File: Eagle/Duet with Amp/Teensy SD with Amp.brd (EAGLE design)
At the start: 34.3 x 63.2 mm, 20 parts, among them IC1 LM386N-4

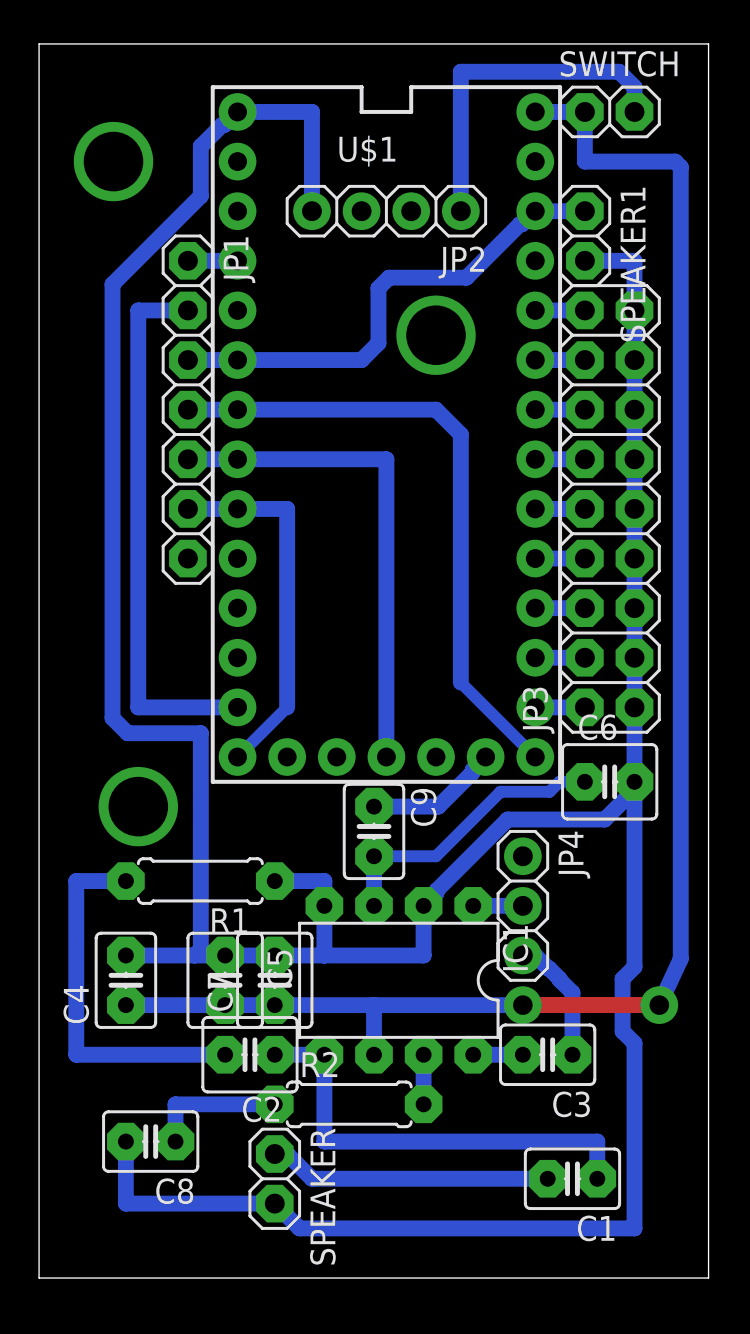
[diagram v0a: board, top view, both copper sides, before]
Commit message: Traced to 32mils
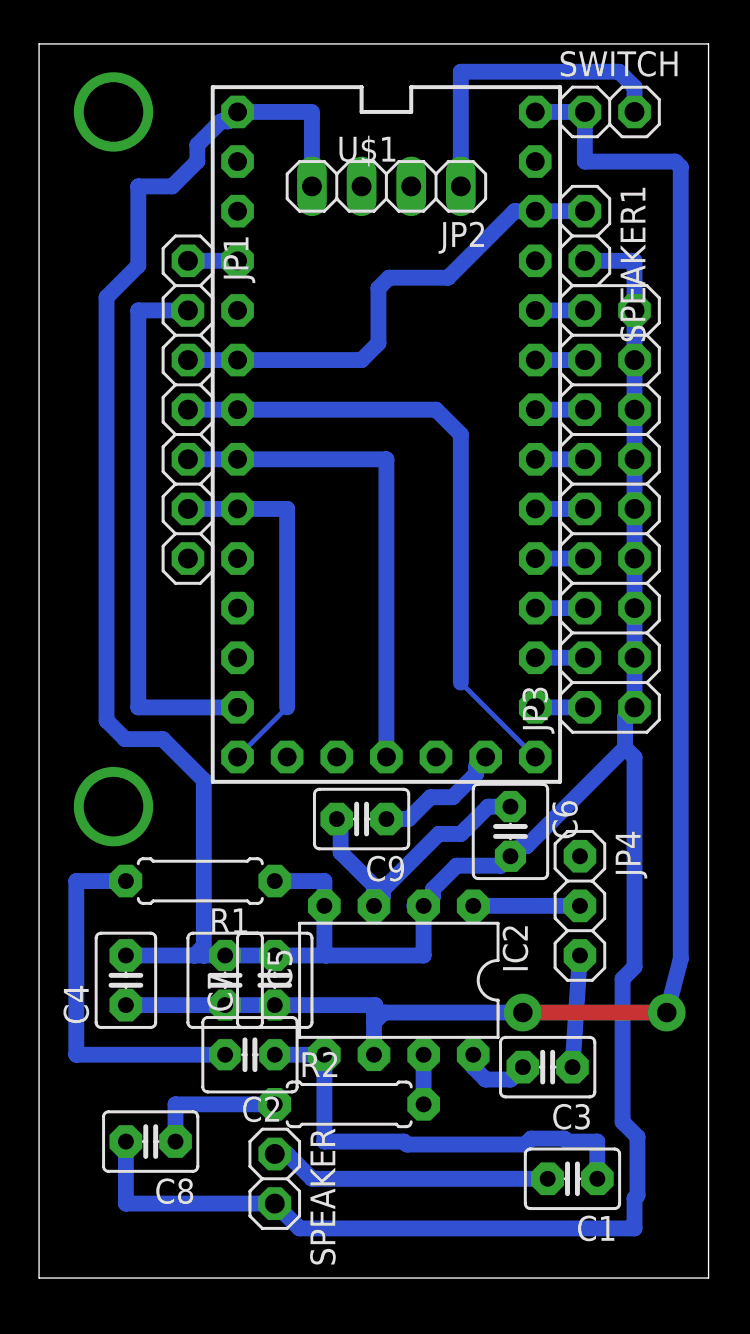
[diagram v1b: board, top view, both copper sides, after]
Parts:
- IC2: value LM386N-4 -> LM386N-1
- moved C6 5.68 mm to (24.1, 22.9), turned to 270 degrees
- moved JP4 2.92 mm to (27.7, 19.1)
- moved JP2 1.27 mm to (17.8, 55.9)
- moved C9 0.90 mm to (16.5, 23.5), turned to 180 degrees
- moved C3 0.63 mm to (26.0, 10.8)
- renumbered IC1 to IC2
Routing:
- net N$26: track 2.54 -> 5.46 mm
- net GND: track 204.2 -> 205.7 mm
- net N$2: track 2.54 -> 3.70 mm
- net N$1: track 6.53 -> 5.73 mm
- net N$6: track 14.9 -> 15.5 mm

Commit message: Revert "Traced to 32mils"
This reverts commit ffbe95997752b5ed6823b856a1fed8613c21e4f0.
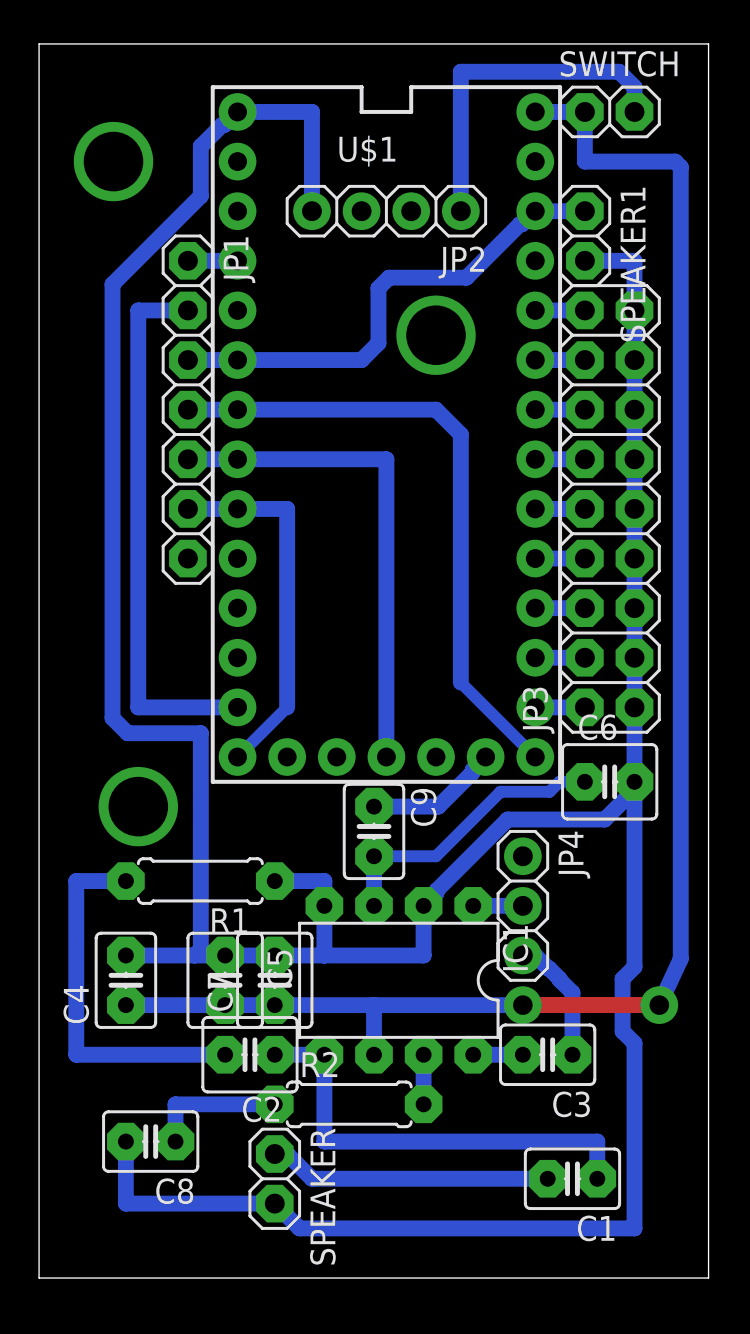
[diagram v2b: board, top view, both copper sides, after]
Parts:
- IC1: value LM386N-1 -> LM386N-4
- moved C6 5.68 mm to (29.2, 25.4), turned to 0 degrees
- moved JP4 2.92 mm to (24.8, 19.1)
- moved JP2 1.27 mm to (17.8, 54.6)
- moved C9 0.90 mm to (17.1, 22.9), turned to 270 degrees
- moved C3 0.63 mm to (26.0, 11.4)
- renumbered IC2 to IC1
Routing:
- net N$26: track 5.46 -> 2.54 mm
- net GND: track 205.7 -> 204.2 mm
- net N$2: track 3.70 -> 2.54 mm
- net N$1: track 5.73 -> 6.53 mm
- net N$6: track 15.5 -> 14.9 mm
